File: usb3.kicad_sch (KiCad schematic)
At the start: 50 parts, among them J5 WE_632723300011_alt_symbol, Q19 PJE138K, Q4 PJE138K, U17 HD3SS3220, U18 AP22615, U19 TPD4E05U06QDQARQ1, U20 TPD4E05U06QDQARQ1, U21 TPD4E05U06QDQARQ1

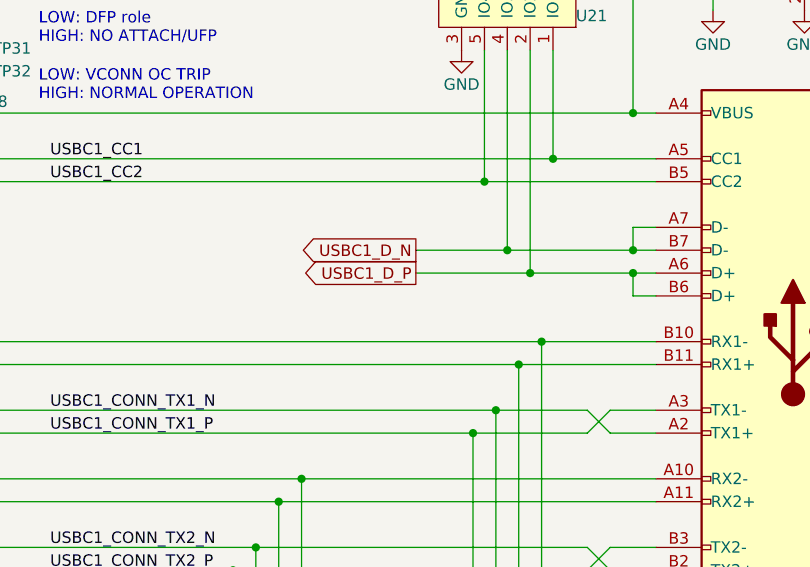
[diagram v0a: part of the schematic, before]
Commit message: Small changes
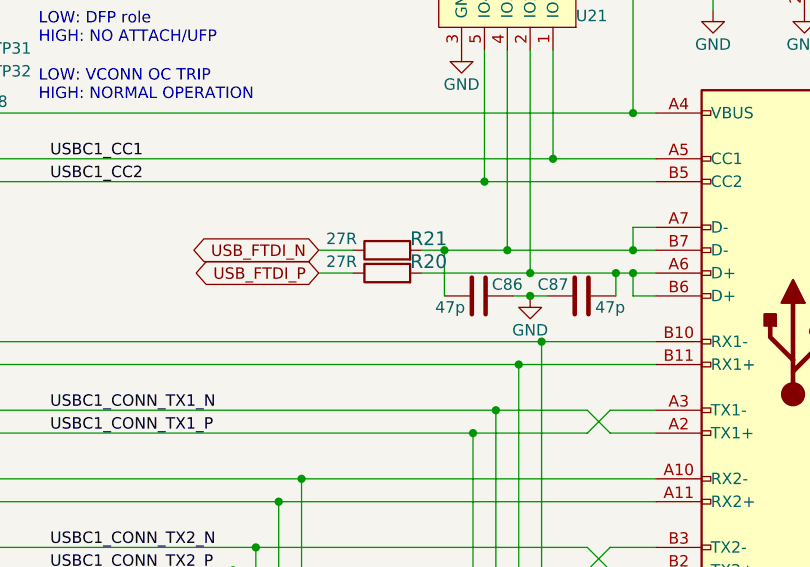
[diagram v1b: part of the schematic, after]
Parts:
- added C86, C87: 47p, symbol Device:C
- added R20, R21: R_27R_0402, jetson-orin-baseboard-footprints:0402-res, symbol jetson-orin-baseboard:R_27R_0402
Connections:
- net GND: now also C86.2, C87.1
- net USBC1_D_N: no longer names the net of J5.A7 (D-), J5.B7 (D-), U21.4 (IO3), U21.7 (IO3)
- net USBC1_D_N: now also C86.1, R21.2
- net USBC1_D_P: no longer names the net of J5.A6 (D+), J5.B6 (D+), U21.2 (IO2), U21.9 (IO2)
- net USBC1_D_P: now also C87.2, R20.2
- new net USB_FTDI_N: R21.1
- new net USB_FTDI_P: R20.1

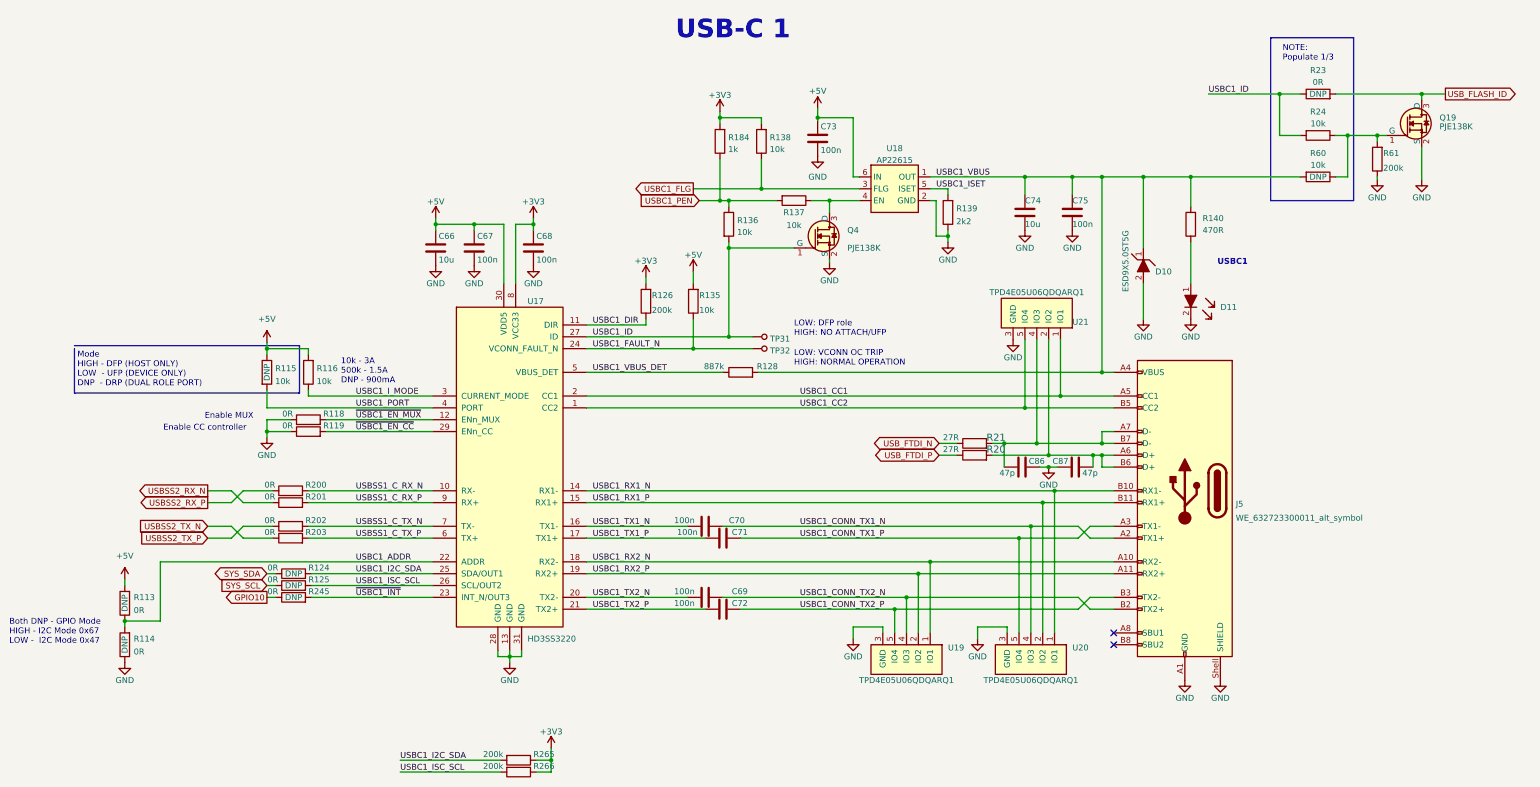
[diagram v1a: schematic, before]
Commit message: Schematic Done
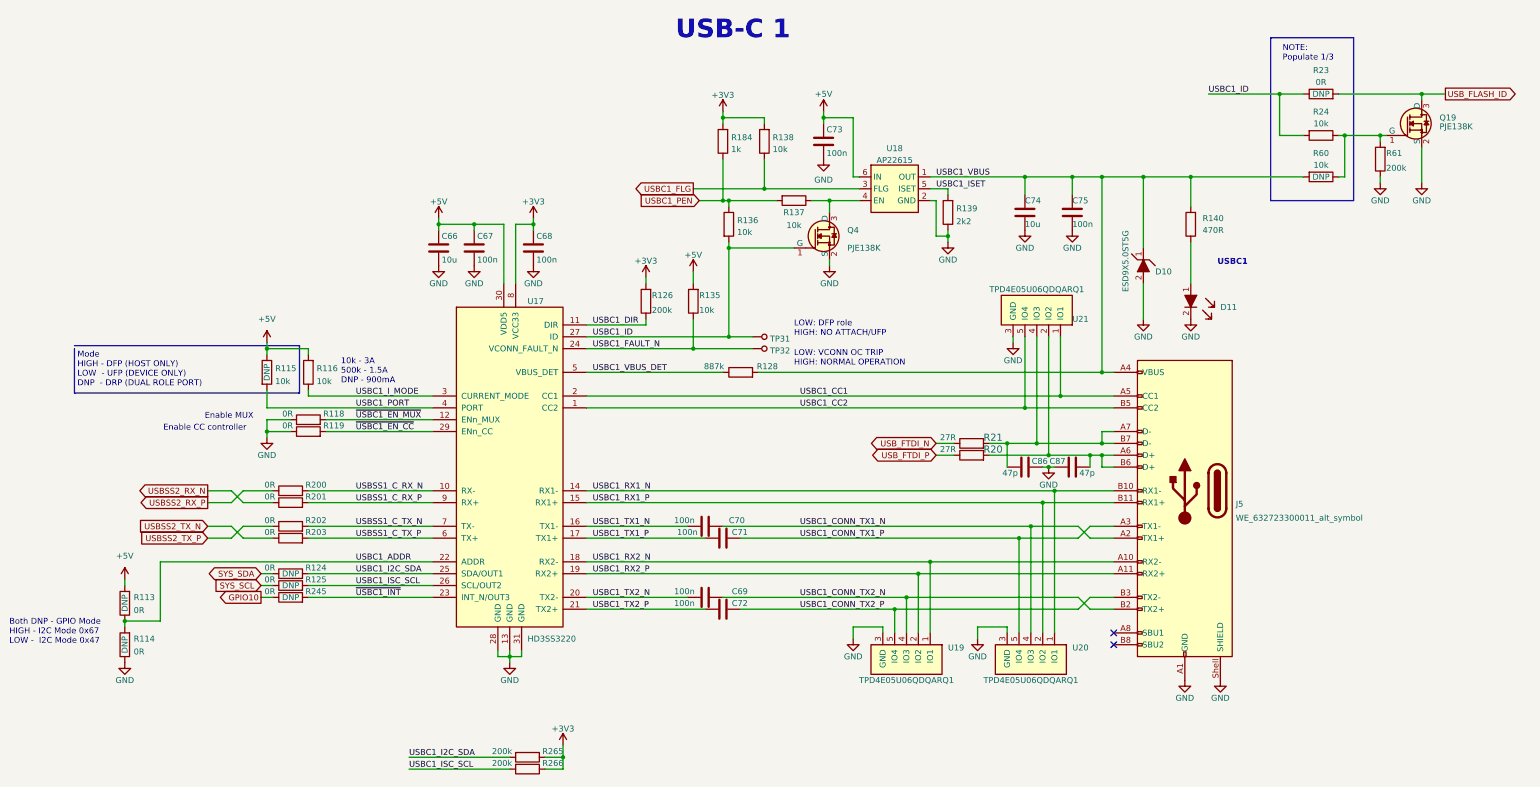
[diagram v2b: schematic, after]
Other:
- moved on the sheet: C66, C73, C86, C87, R124, R125, R138, R184, R20, R21, R23, R24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
